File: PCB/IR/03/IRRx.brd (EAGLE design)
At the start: 64 x 64 mm, 19 parts

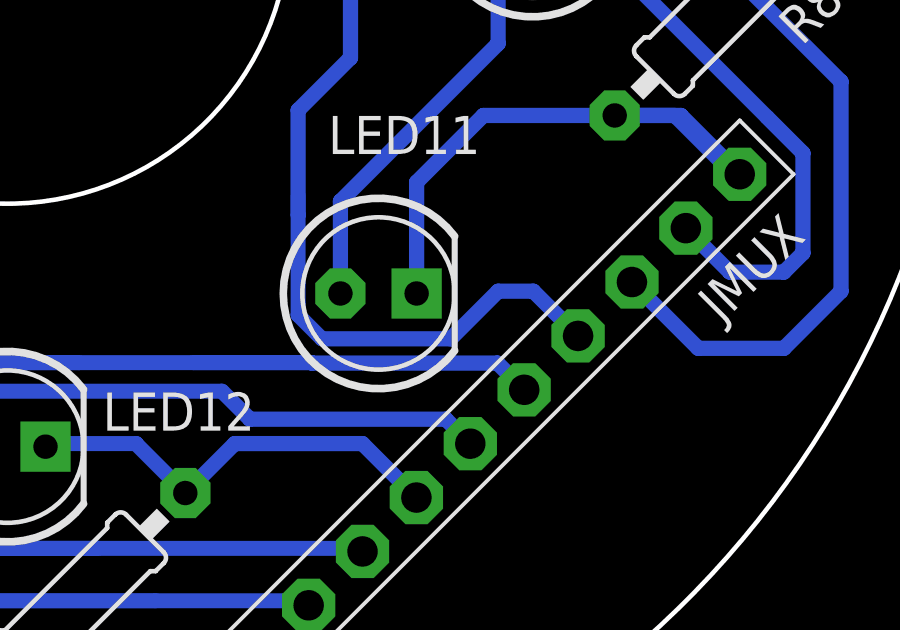
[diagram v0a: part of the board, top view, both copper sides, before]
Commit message: modified IR-TX
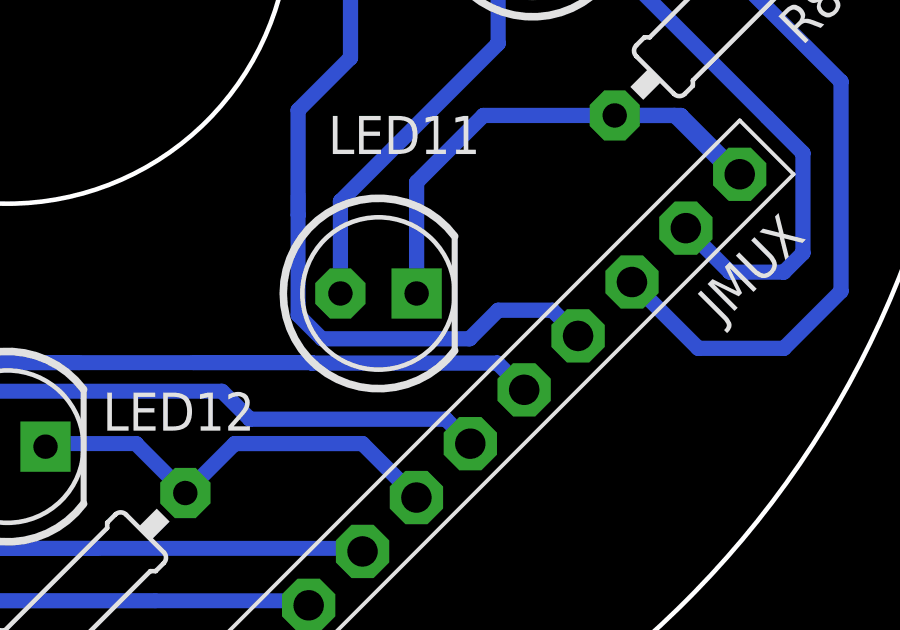
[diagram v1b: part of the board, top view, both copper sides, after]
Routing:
- net N$5: track 49.4 -> 48.9 mm
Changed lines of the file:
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@@
 <setting verticaltext="up"/>
 </settings>
-<grid distance="25" unitdist="mil" unit="mil" style="lines" multiple="1" display="no" altdistance="5" altunitdist="mil" altunit="mil"/>
+<grid distance="25" unitdist="mil" unit="mm" style="lines" multiple="1" display="no" altdistance="5" altunitdist="mil" altunit="mil"/>
 <layers>
 <layer number="1" name="Top" color="4" fill="1" visible="yes" active="yes"/>
@@
 <wire x1="41.43375" y1="27.46375" x2="41.43375" y2="36.83" width="0.508" layer="16"/>
 <wire x1="39.6875" y1="25.7175" x2="41.43375" y2="27.46375" width="0.508" layer="16"/>
-<wire x1="46.355" y1="19.685" x2="47.52815" y2="19.685" width="0.508" layer="16"/>
-<wire x1="47.52815" y1="19.685" x2="49.019075" y2="18.194075" width="0.508" layer="16"/>
-<wire x1="40.48125" y1="18.0975" x2="44.7675" y2="18.0975" width="0.508" layer="16"/>
-<wire x1="44.7675" y1="18.0975" x2="46.355" y2="19.685" width="0.508" layer="16"/>
+<wire x1="46.355" y1="19.05" x2="48.16315" y2="19.05" width="0.508" layer="16"/>
+<wire x1="48.16315" y1="19.05" x2="49.019075" y2="18.194075" width="0.508" layer="16"/>
+<wire x1="40.48125" y1="18.0975" x2="45.4025" y2="18.0975" width="0.508" layer="16"/>
+<wire x1="45.4025" y1="18.0975" x2="46.355" y2="19.05" width="0.508" layer="16"/>
 </signal>
 <signal name="N$6">
